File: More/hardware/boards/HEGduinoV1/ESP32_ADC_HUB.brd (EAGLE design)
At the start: 71.9 x 30 mm, 8 parts

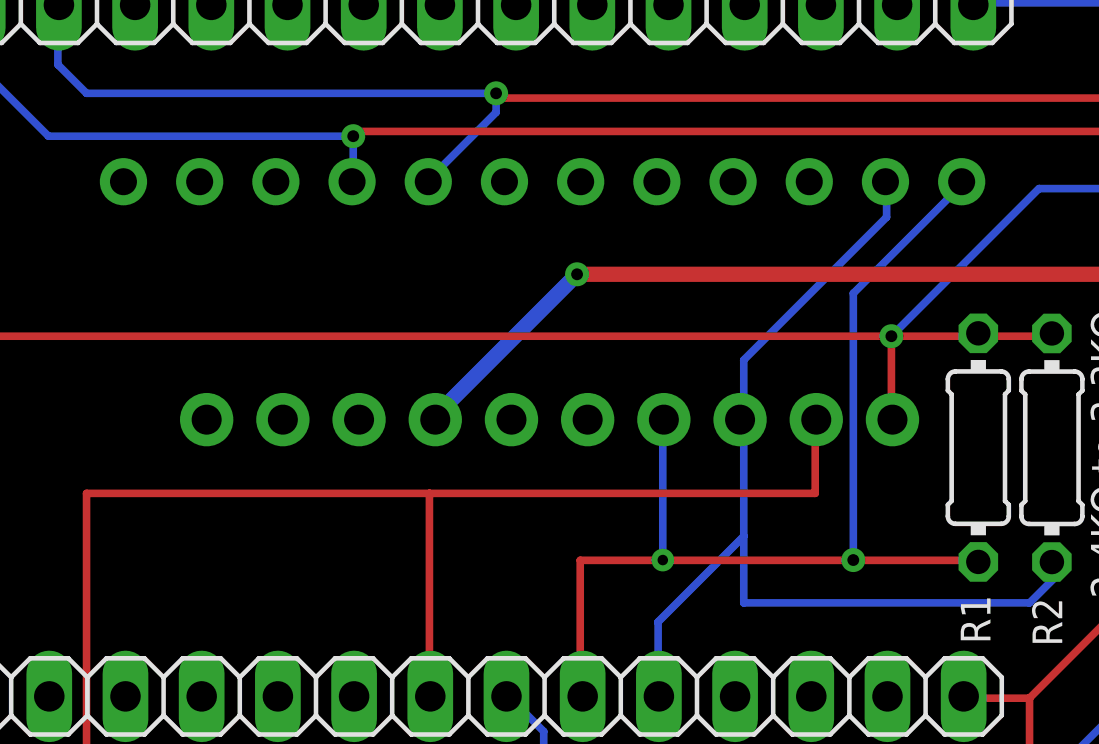
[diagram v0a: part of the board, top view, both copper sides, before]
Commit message: Added some sensor designs, moved some stuff
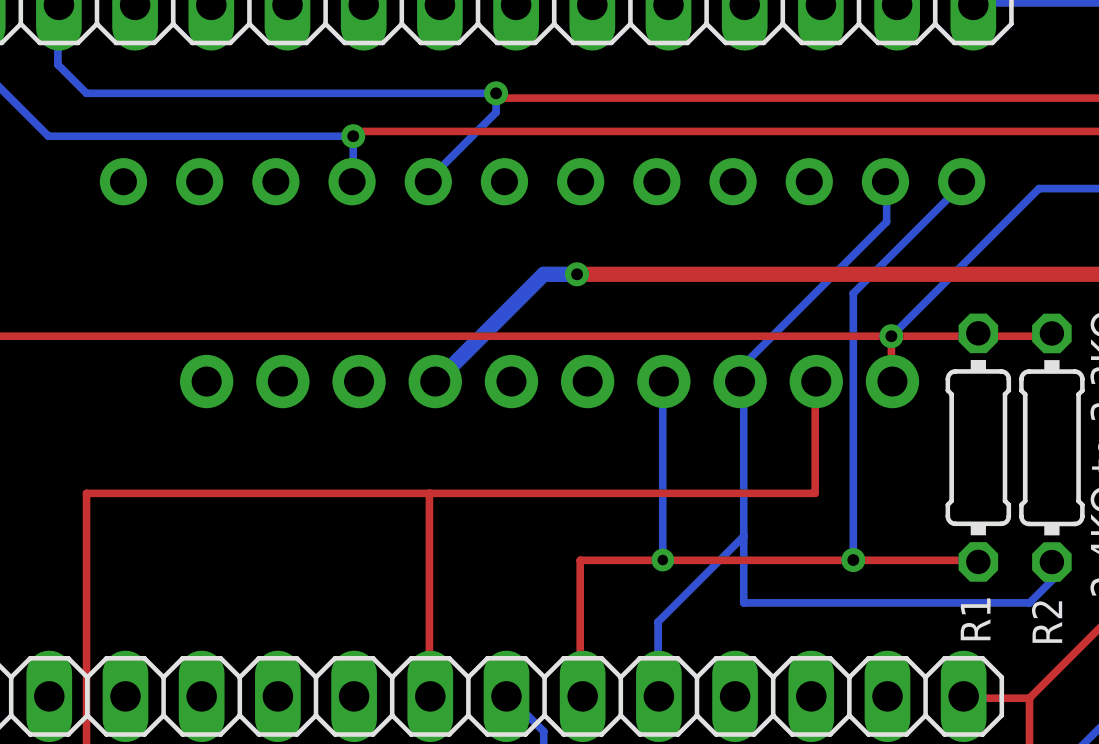
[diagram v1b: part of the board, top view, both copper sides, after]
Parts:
- moved ADS1115 1.27 mm to (40.0, 38.5)
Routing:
- net ADC_GND: track 44.0 -> 45.4 mm
- net SDA: track 36.6 -> 37.9 mm
- net VBAT: track 89.8 -> 88.7 mm
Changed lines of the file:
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@@
 <attribute name="VALUE" x="55.047590625" y="28.01005" size="0.4064" layer="27" ratio="10" rot="R180"/>
 </element>
-<element name="ADS1115" library="microbuilder" package="1X10_ROUND70" value="" x="40.040815625" y="37.223853125" smashed="yes" rot="R180">
-<attribute name="NAME" x="27.298803125" y="39.482015625" size="0.8128" layer="26" ratio="10" rot="MR270"/>
-<attribute name="VALUE" x="52.740815625" y="40.398853125" size="0.8128" layer="27" rot="R180"/>
+<element name="ADS1115" library="microbuilder" package="1X10_ROUND70" value="" x="40.040815625" y="38.493853125" smashed="yes" rot="R180">
+<attribute name="NAME" x="27.298803125" y="40.752015625" size="0.8128" layer="26" ratio="10" rot="MR270"/>
+<attribute name="VALUE" x="52.740815625" y="41.668853125" size="0.8128" layer="27" rot="R180"/>
 </element>
 <element name="R1" library="resistor" library_urn="urn:adsk.eagle:library:348" package="0204/7" package3d_urn="urn:adsk.eagle:package:23498/1" value="" x="54.3327375" y="36.29111875" smashed="yes" rot="R270">
@@
 </signal>
 <signal name="VBAT">
-<wire x1="51.435" y1="40.005" x2="51.435" y2="37.1475" width="0.254" layer="1"/>
+<wire x1="51.435" y1="40.005" x2="51.435" y2="38.25875" width="0.254" layer="1"/>
 <wire x1="51.435" y1="40.005" x2="56.8325" y2="40.005" width="0.254" layer="1"/>
 <wire x1="51.435" y1="40.005" x2="19.52625" y2="40.005" width="0.254" layer="1"/>
@@
 <wire x1="50.165" y1="32.54375" x2="50.165" y2="41.43375" width="0.254" layer="16"/>
 <wire x1="50.165" y1="41.43375" x2="53.81625" y2="45.085" width="0.254" layer="16"/>
-<wire x1="43.815" y1="37.1475" x2="43.815" y2="32.54375" width="0.254" layer="16"/>
+<wire x1="43.815" y1="38.4175" x2="43.815" y2="32.54375" width="0.254" layer="16"/>
 <via x="43.815" y="32.54375" extent="1-16" drill="0.35"/>
 <wire x1="54.169665625" y1="32.534453125" x2="50.165" y2="32.54375" width="0" layer="19" extent="1-1"/>
-<wire x1="43.815" y1="32.54375" x2="41.062909375" y2="32.534453125" width="0" layer="19" extent="1-16"/>
+<wire x1="43.815" y1="32.54375" x2="41.062909375" y2="27.67456875" width="0" layer="19" extent="1-1"/>
 </signal>
 <signal name="SCL">
 <wire x1="46.51375" y1="31.115" x2="56.03875" y2="31.115" width="0.254" layer="16"/>
-<wire x1="46.51375" y1="39.21125" x2="46.51375" y2="33.3375" width="0.254" layer="16"/>
+<wire x1="46.51375" y1="39.0525" x2="46.51375" y2="33.3375" width="0.254" layer="16"/>
 <wire x1="46.51375" y1="33.3375" x2="43.65625" y2="30.48" width="0.254" layer="16"/>
 <wire x1="43.65625" y1="30.48" x2="43.65625" y2="27.6225" width="0.254" layer="16"/>
 <wire x1="46.51375" y1="33.3375" x2="46.51375" y2="31.115" width="0.254" layer="16"/>
-<wire x1="46.51375" y1="39.21125" x2="51.27625" y2="43.97375" width="0.254" layer="16"/>
-<wire x1="51.27625" y1="43.97375" x2="51.27625" y2="45.085" width="0.254" layer="16"/>
+<wire x1="46.51375" y1="39.0525" x2="51.27625" y2="43.815" width="0.254" layer="16"/>
+<wire x1="51.27625" y1="43.815" x2="51.27625" y2="45.085" width="0.254" layer="16"/>
 <wire x1="56.03875" y1="31.115" x2="56.8325" y2="31.90875" width="0.254" layer="16"/>
 <wire x1="56.8325" y1="31.90875" x2="56.8325" y2="32.385" width="0.254" layer="16"/>
@@
 </signal>
 <signal name="A0">
-<wire x1="40.9575" y1="42.06875" x2="36.195" y2="37.30625" width="0.508" layer="16"/>
+<wire x1="40.9575" y1="42.06875" x2="39.84625" y2="42.06875" width="0.508" layer="16"/>
+<wire x1="39.84625" y1="42.06875" x2="36.195" y2="38.4175" width="0.508" layer="16"/>
 <via x="40.9575" y="42.06875" extent="1-16" drill="0.3937"/>
 <wire x1="40.9575" y1="42.06875" x2="60.0075" y2="42.06875" width="0.508" layer="1"/>
@@
 <wire x1="24.60625" y1="26.035" x2="24.60625" y2="34.76625" width="0.254" layer="1"/>
 <wire x1="24.60625" y1="34.76625" x2="36.03625" y2="34.76625" width="0.254" layer="1"/>
-<wire x1="48.895" y1="34.76625" x2="48.895" y2="37.1475" width="0.254" layer="1"/>
+<wire x1="48.895" y1="34.76625" x2="48.895" y2="38.57625" width="0.254" layer="1"/>
 <wire x1="23.33625" y1="24.92375" x2="23.495" y2="24.92375" width="0.254" layer="1"/>
 <wire x1="23.495" y1="24.92375" x2="24.60625" y2="26.035" width="0.254" layer="1"/>
